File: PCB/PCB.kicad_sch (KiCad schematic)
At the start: 20 parts, among them U1 STM32G031F6P6, U2 A7106, U3 HT7333-3.3V, Y1 16MHz

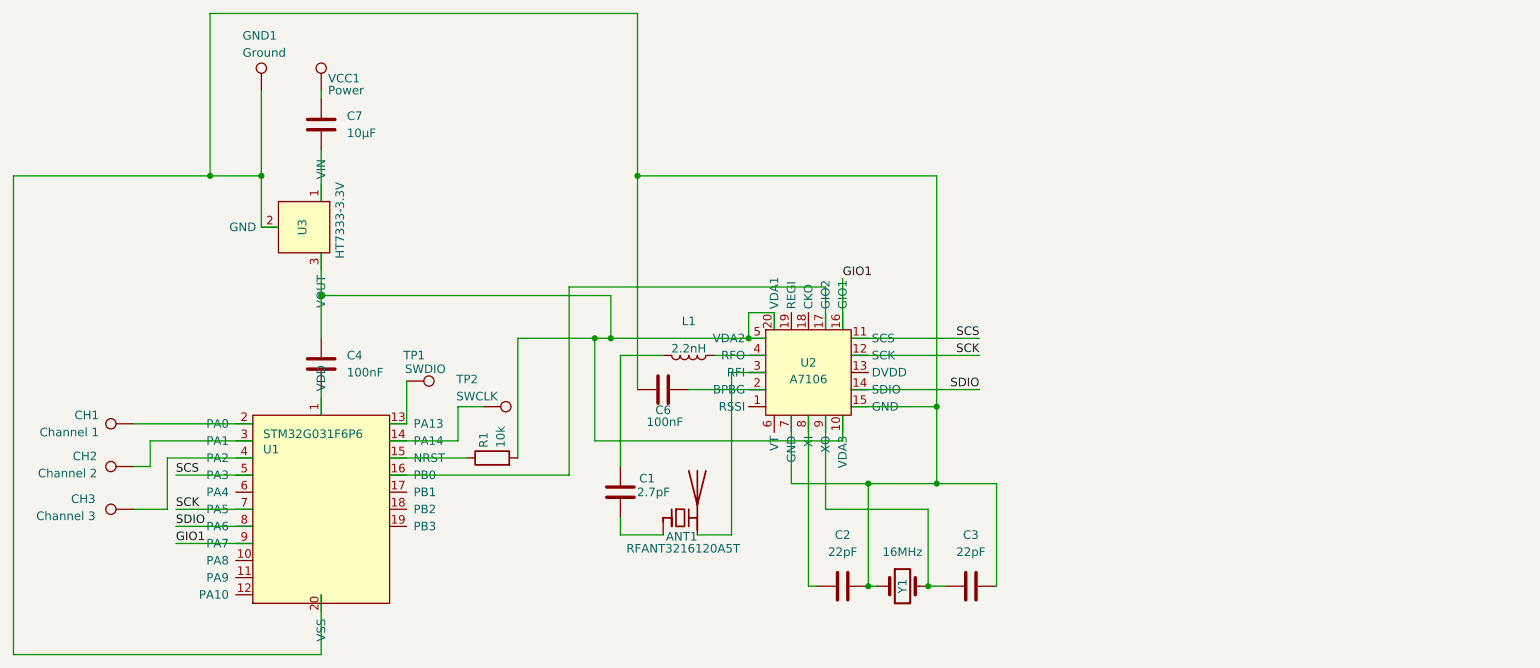
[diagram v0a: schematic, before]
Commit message: Organise the schematic
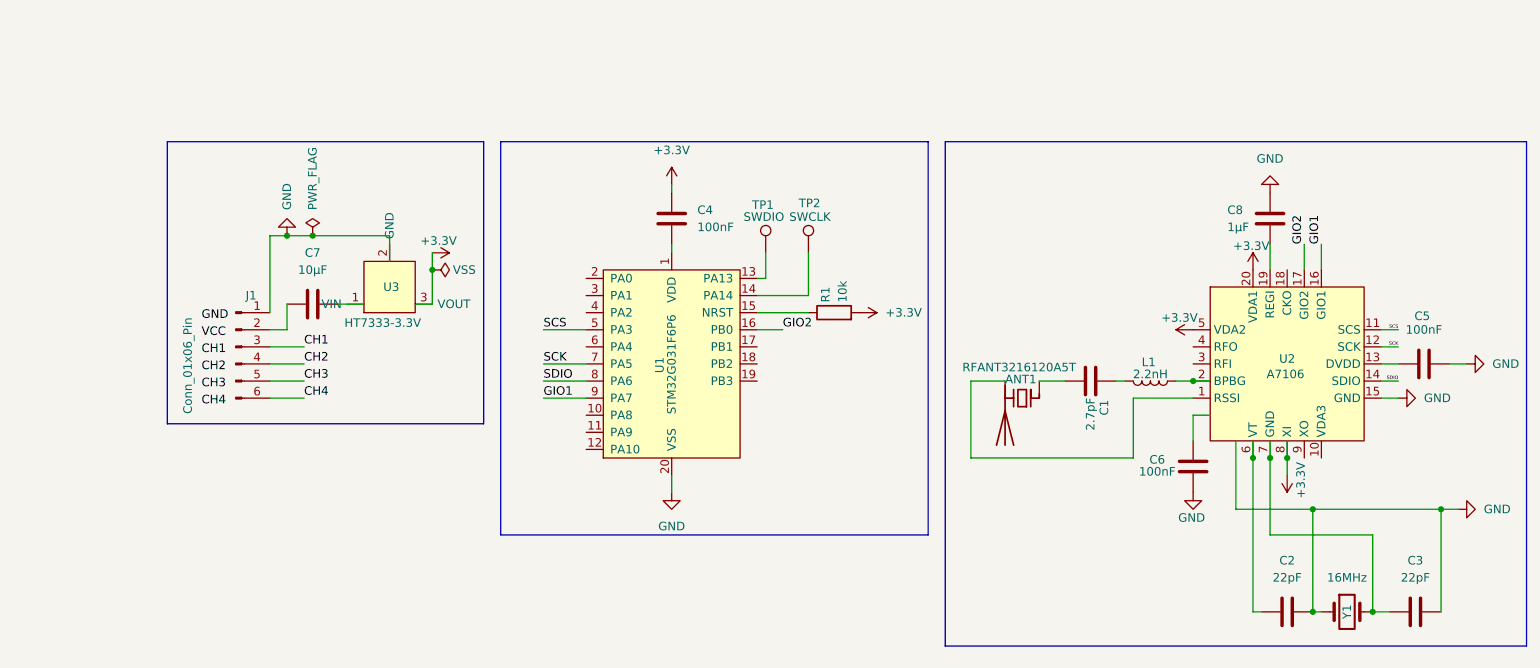
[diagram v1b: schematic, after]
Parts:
- removed CH1: Channel 1, TestPoint:TestPoint_THTPad_1.0x1.0mm_Drill0.5mm, symbol Connector:TestPoint
- removed CH2: Channel 2, TestPoint:TestPoint_THTPad_1.0x1.0mm_Drill0.5mm, symbol Connector:TestPoint
- removed CH3: Channel 3, TestPoint:TestPoint_THTPad_1.0x1.0mm_Drill0.5mm, symbol Connector:TestPoint
- removed GND1: Ground, TestPoint:TestPoint_THTPad_1.0x1.0mm_Drill0.5mm, symbol Connector:TestPoint
- removed VCC1: Power, TestPoint:TestPoint_THTPad_1.0x1.0mm_Drill0.5mm, symbol Connector:TestPoint
- added C5: 100nF, Capacitor_SMD:C_0402_1005Metric, symbol Device:C
- added C8: 1µF, symbol Device:C
- added J1: Conn_01x06_Pin, Connector_PinHeader_2.54mm:PinHeader_1x06_P2.54mm_Vertical, symbol Connector:Conn_01x06_Pin
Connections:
- net GND: now reaches C2.2, C3.2, C6.1, U1.20 (VSS), U2.15 (GND), U3.2 (GND), Y1.1
- net GND: now also C5.1, C8.1, J1.1 (Pin_1); no longer U2.7 (GND)
- net at C6.2: no longer U2.2 (BPBG)
- net at C7.1: now also J1.2 (Pin_2)
- net at U2.1 (RSSI): now also ANT1.2 (PCB_Trace)
- net +3.3V: now reaches C4.1, R1.2, U2.20 (VDA1), U2.5 (VDA2), U3.3 (VOUT)
- net +3.3V: now also U2.8 (XI); no longer U2.10 (VDA3)
- net at U2.13 (DVDD): now also C5.2
- net GIO2: now reaches U1.16 (PB0), U2.17 (GIO2)
- net at U2.19 (REGI): now also C8.2
- net at U2.3 (RFI): no longer ANT1.2 (PCB_Trace)
- net at L1.1: now also U2.2 (BPBG); no longer U2.4 (RFO)
- net at U2.6 (VT): now also C2.1
- net at C3.1, Y1.2: now also U2.7 (GND); no longer U2.9 (XO)
- new net CH1: J1.3 (Pin_3)
- new net CH2: J1.4 (Pin_4)
- new net CH3: J1.5 (Pin_5)
- new net CH4: J1.6 (Pin_6)
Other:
- moved on the sheet: ANT1, C1, C2, C3, C4, C6, C7, L1, R1, TP1, TP2, U1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
